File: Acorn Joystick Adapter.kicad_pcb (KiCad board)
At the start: 2 copper layers, 67.9 x 52.1 mm, 32 parts, among them J1 Acorn Computer, J2 Atari #1, J3 Atari #2, J4 Analog, Q1 BC337, Q2 BC337, Q3 BC337, Q4 BC337, Q5 BC337, Q6 BC337

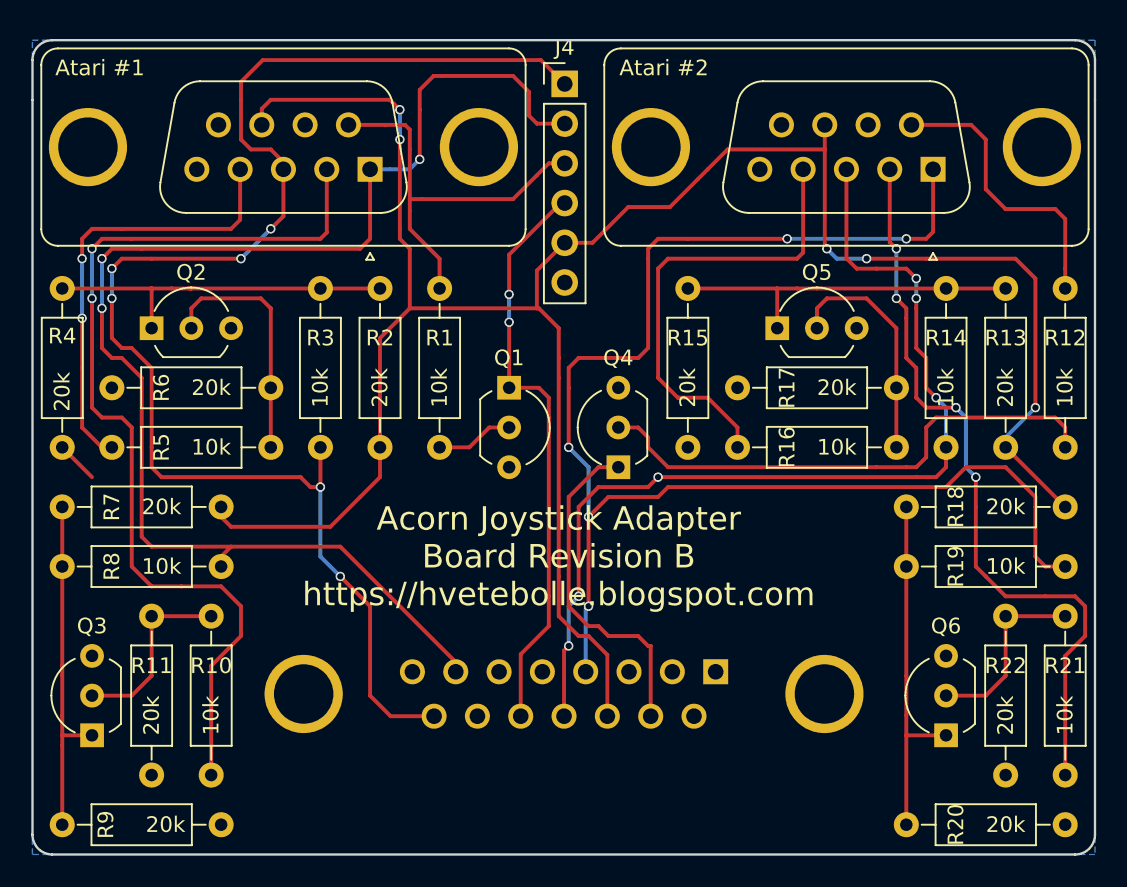
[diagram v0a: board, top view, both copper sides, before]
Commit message: Upgrade schematic to new KiCAD
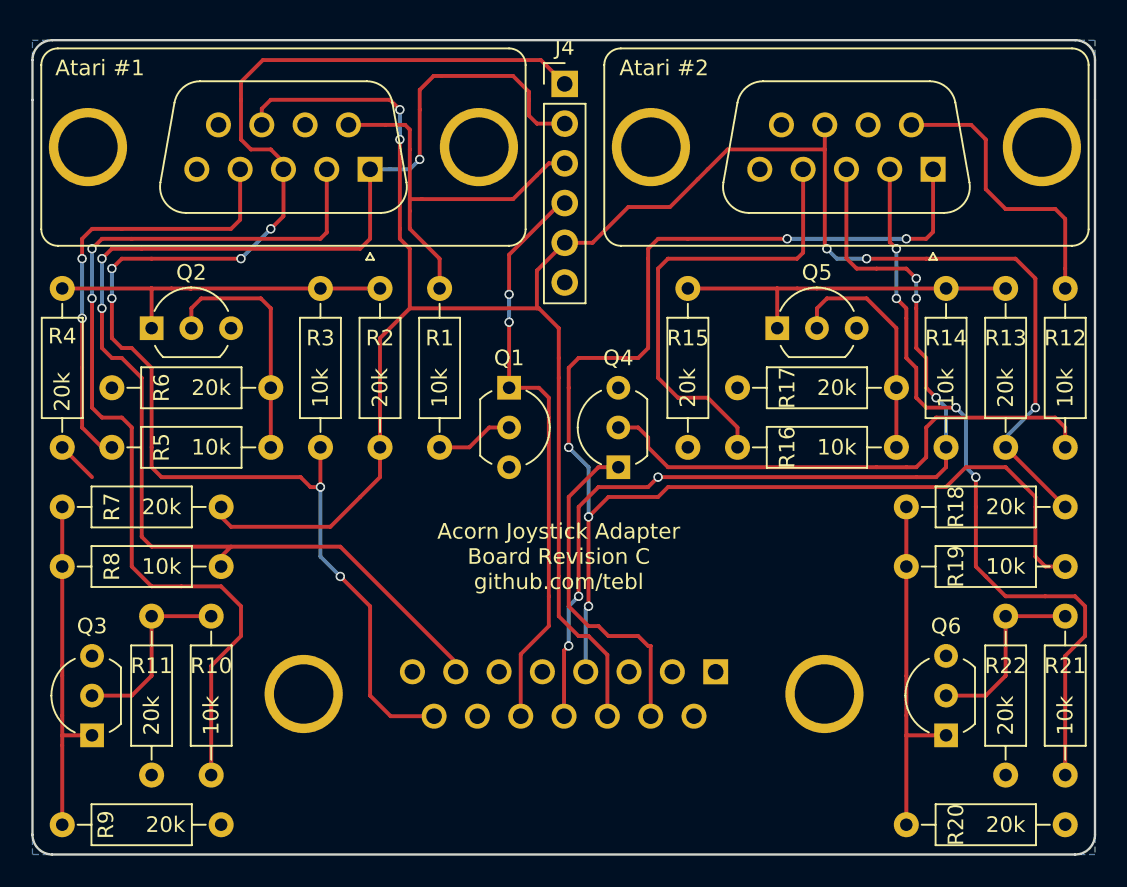
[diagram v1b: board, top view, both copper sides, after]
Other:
- net class Default removed
- board text added: "Acorn Joystick Adapter"
- board text added: "Acorn Joystick Adapter Board Revision C github.com/tebl"
- board text removed: "Acorn Joystick Adapter Board Revision B"
- board text removed: "Acorn Joystick Adapter Board Revision B https://hvetebolle.blogspot.com"
